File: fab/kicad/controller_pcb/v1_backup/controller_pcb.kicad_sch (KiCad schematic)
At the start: 62 parts, among them J1 Screw_Terminal_01x04, J10 1935161, J11 Screw_Terminal_01x06, J2 Screw_Terminal_01x03, J3 Screw_Terminal_01x03, J4 Screw_Terminal_01x03, J5 Screw_Terminal_01x06, J6 Screw_Terminal_01x06, J7 Screw_Terminal_01x02, J8 1935161, J9 Screw_Terminal_01x02, Q1 IRLZ44N, U1 TPS55289RYQR, U2 TPS55289RYQR, U3 DS3231SN, U4 BK-912-TR

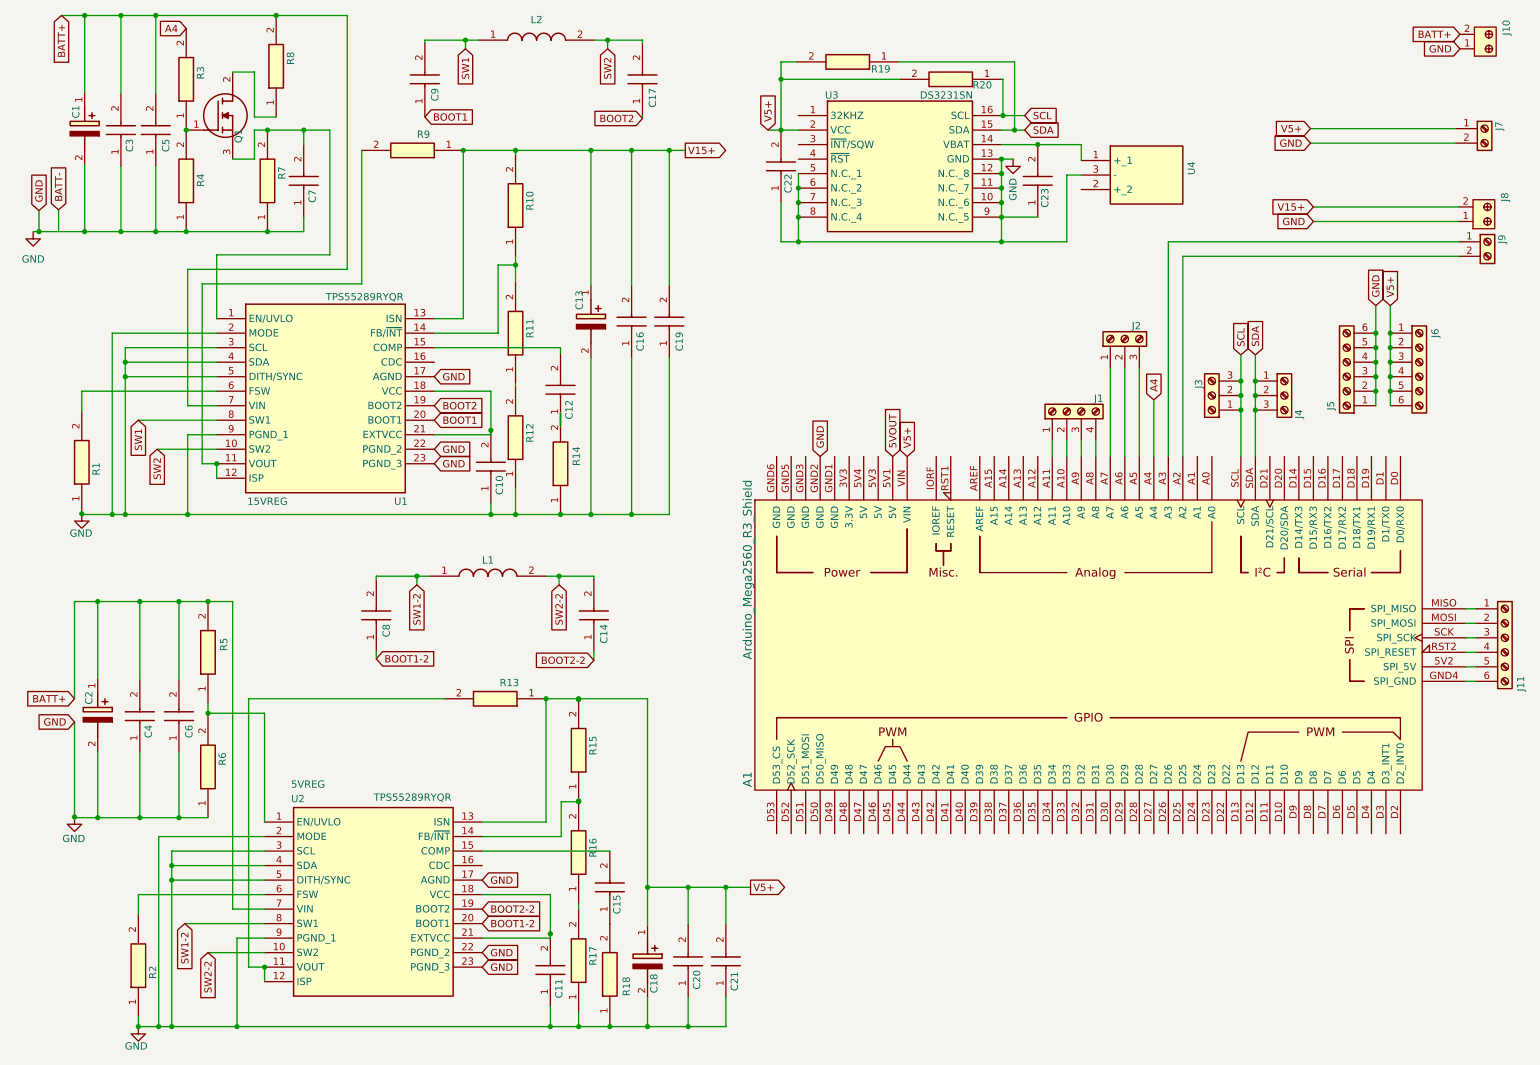
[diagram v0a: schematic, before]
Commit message: v2 of PCB
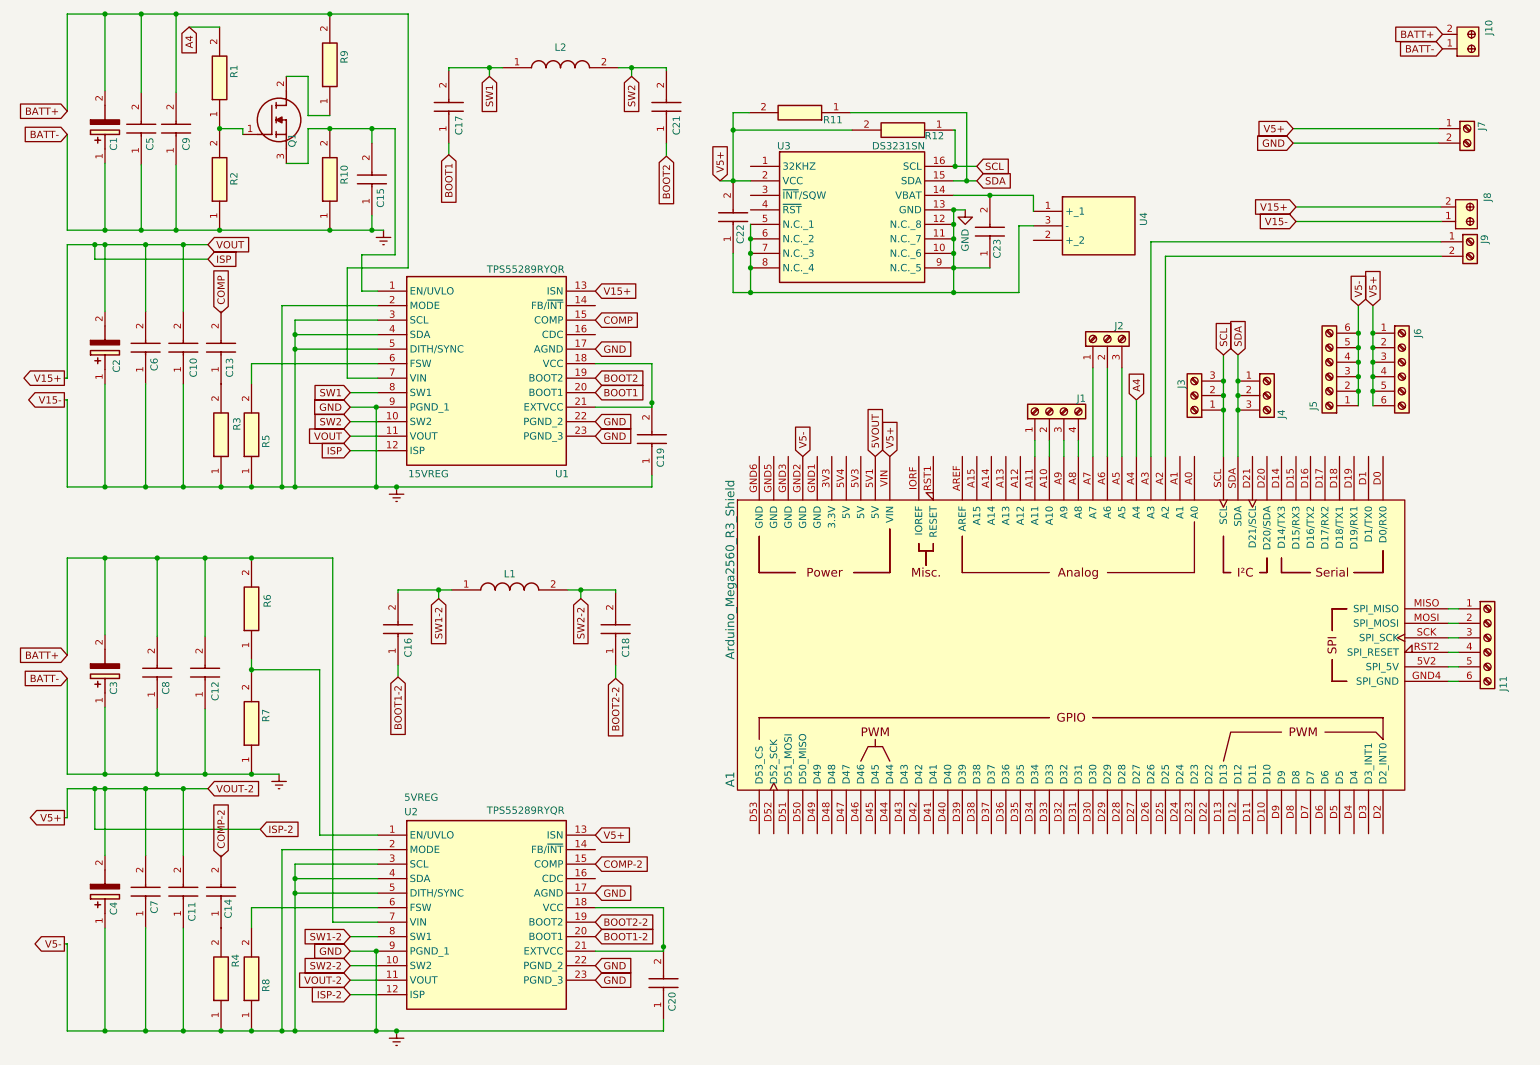
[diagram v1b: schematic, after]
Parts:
- removed R10, R15: CRCW0402100KFKED, extracted:RESC1005X40N, symbol CRCW0402100KFKED:CRCW0402100KFKED
- removed R11: CFM14JT8K20, Resistor_THT:R_Axial_DIN0204_L3.6mm_D1.6mm_P5.08mm_Horizontal, symbol CRCW0402100KFKED:CRCW0402100KFKED
- removed R12: MBA02040C7320FRP00, Resistor_THT:R_Axial_DIN0204_L3.6mm_D1.6mm_P5.08mm_Horizontal, symbol CRCW0402100KFKED:CRCW0402100KFKED
- removed R13, R9: WLBR050FET, Resistor_THT:R_Axial_DIN0411_L9.9mm_D3.6mm_P12.70mm_Horizontal, symbol CRCW0402100KFKED:CRCW0402100KFKED
- removed R16: RN55D3202FB14, Resistor_THT:R_Axial_DIN0207_L6.3mm_D2.5mm_P7.62mm_Horizontal, symbol CRCW0402100KFKED:CRCW0402100KFKED
- removed R17: CF14JT620R, Resistor_THT:R_Axial_DIN0207_L6.3mm_D2.5mm_P7.62mm_Horizontal, symbol CRCW0402100KFKED:CRCW0402100KFKED
- renumbered C19 to C10, C21 to C11, C6 to C12, C12 to C13, C15 to C14, C7 to C15, C8 to C16, C9 to C17, C14 to C18, C10 to C19, C13 to C2, C11 to C20, C17 to C21, C2 to C3, C18 to C4, C3 to C5, C16 to C6, C20 to C7, C4 to C8, C5 to C9, R3 to R1, R7 to R10, R19 to R11, R20 to R12, R4 to R2, R14 to R3, R18 to R4, R1 to R5, R5 to R6, R6 to R7, R2 to R8, R8 to R9
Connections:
- net BATT+: now also C1.2, C3.2; no longer C1.1 (K), C3.1 (K)
- net ISP: now reaches U1.11 (VOUT), U1.12 (ISP)
- net ISP: now also C10.2, C2.2 (-), C6.2, J8.2, U1.13 (ISN)
- net COMP: now reaches C13.2, U1.15 (COMP)
- net COMP-2: now reaches C14.2, U2.15 (COMP)
- net ISP-2: now reaches U2.11 (VOUT), U2.12 (ISP)
- net ISP-2: now also A1.VIN, C11.2, C22.2, C4.2 (-), C7.2, J6.1 (Pin_1), J6.2 (Pin_2), J6.3 (Pin_3), J6.4 (Pin_4), J6.5 (Pin_5), J6.6 (Pin_6), J7.1 (Pin_1), R11.2, R12.2, U2.13 (ISN), U3.2 (VCC)
- net GND renamed Earth
- net Earth: now also C1.1 (K), C2.1 (+), C3.1 (K), C4.1 (+); no longer C1.2, C2.2 (-), C3.2, C4.2 (-)
- removed net V15+: C10.2, C2.1 (+), C6.2, J8.2, U1.13 (ISN)
- removed net V5+: A1.VIN, C11.2, C22.2, C4.1 (+), C7.2, J6.1 (Pin_1), J6.2 (Pin_2), J6.3 (Pin_3), J6.4 (Pin_4), J6.5 (Pin_5), J6.6 (Pin_6), J7.1 (Pin_1), R11.2, R12.2, U2.13 (ISN), U3.2 (VCC)
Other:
- moved on the sheet: A1, C1, C10, C11, C12, C13, C14, C15, C16, C17, C18, C19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
